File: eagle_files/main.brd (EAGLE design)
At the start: 45.4 x 40.6 mm, 9 parts, among them X1 22-23-2021

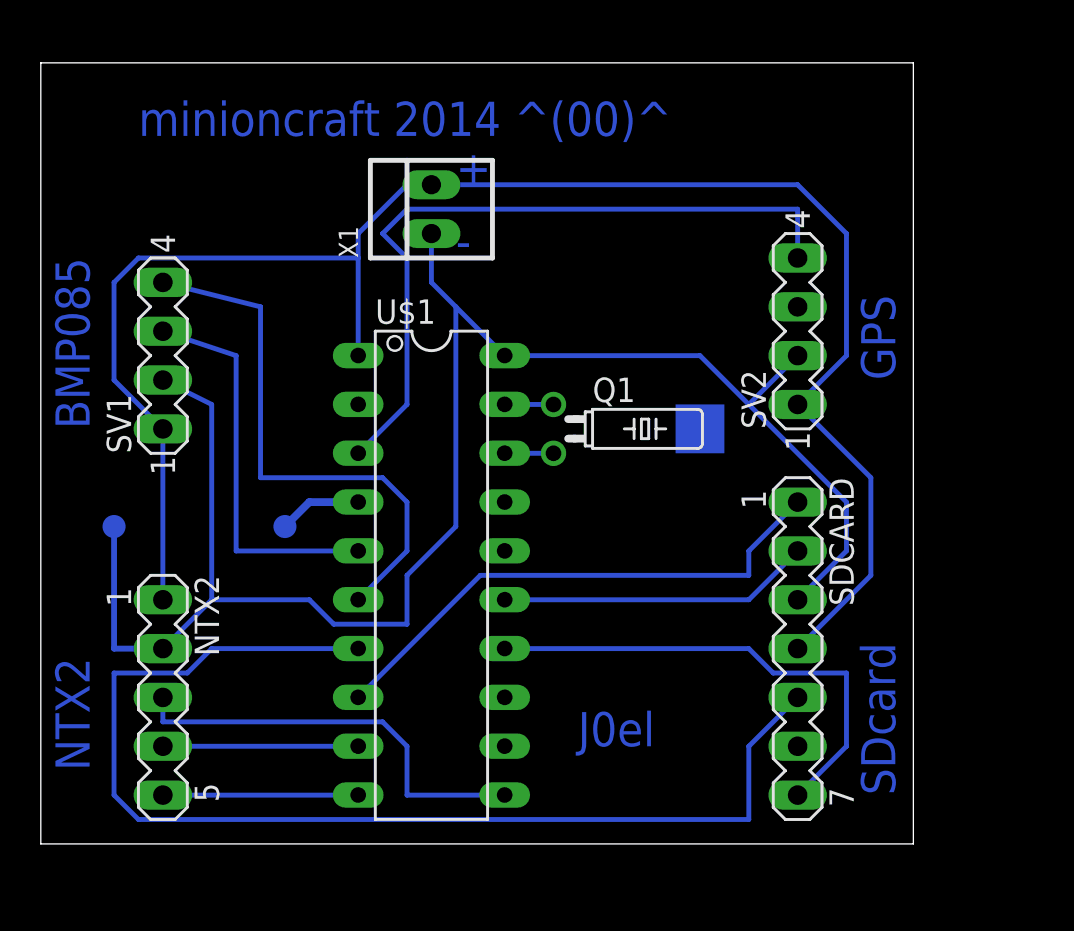
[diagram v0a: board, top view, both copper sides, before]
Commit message: fix board design
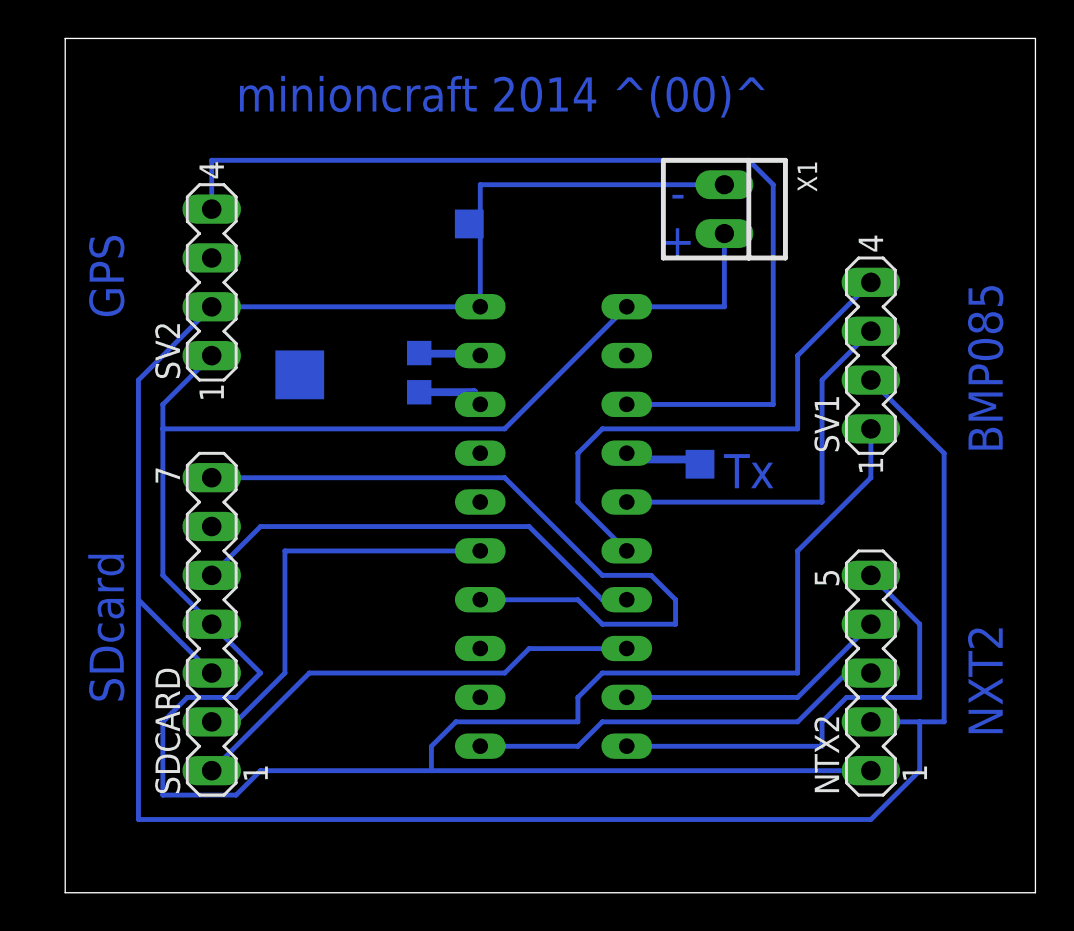
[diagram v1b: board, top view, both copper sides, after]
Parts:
- removed Q1: (no value), crystal:TC26H
- removed TP1, TP2: TPTP12R, testpad:TP12R
- moved NTX2 36.9 mm to (40.6, 8.89), turned to 90 degrees
- moved SV1 36.8 mm to (40.6, 25.4)
- moved SV2 30.6 mm to (6.35, 29.2)
- moved SDCARD 30.5 mm to (6.35, 11.4), turned to 90 degrees
- moved X1 15.2 mm to (33.0, 33.0), turned to 270 degrees
- moved U$1 6.84 mm to (24.1, 16.5), flipped to the bottom
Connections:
- removed net N$14: TP1.TP
- net GND: no longer TP2.TP
- net N$10: no longer Q1.1
- net N$12: no longer Q1.2
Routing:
- net +3V3: track 90.4 -> 139.5 mm
- net GND: track 92.3 -> 134.1 mm
- net N$5: track 60.5 -> 24.2 mm
- net N$8: track 10.2 -> 24.4 mm
- net N$7: track 37.7 -> 51.3 mm
- net N$6: track 25.7 -> 38.7 mm
- net N$4: track 16.3 -> 21.4 mm
- net N$11: track 10.2 -> 14.3 mm
- net N$14: track 0.00 -> 3.71 mm
- net N$3: track 27.8 -> 24.2 mm
- net N$15: track 0.00 -> 3.00 mm
- net N$12: track 2.54 -> 0.00 mm
- net N$10: track 2.54 -> 0.01 mm
- net N$1: track 28.4 -> 27.3 mm
- net N$13: track 4.34 -> 3.50 mm
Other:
- board size 45.4 x 40.6 mm -> 50.5 x 44.4 mm
- board text added: "NXT2"
- board text added: "Tx"
- board text removed: "J0el"
- board text removed: "NTX2"
